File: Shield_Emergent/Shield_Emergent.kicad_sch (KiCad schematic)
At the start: 18 parts, among them J1 Conn_01x02_Female, J3 Conn_01x02_Female, J5 Conn_02x06_Odd_Even, U1 Raspberri_Pi_Pico, U2 TPS2553, U3 TPS2553

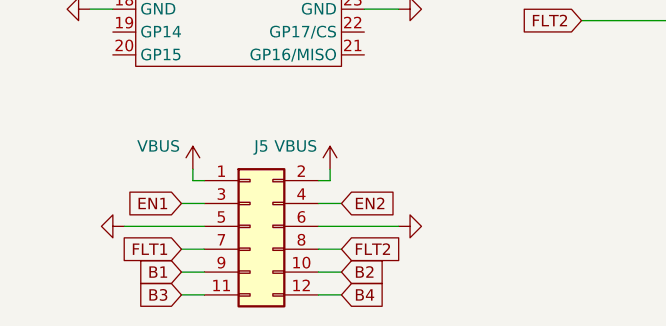
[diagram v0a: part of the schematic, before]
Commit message: v1.7 DRC was conducted
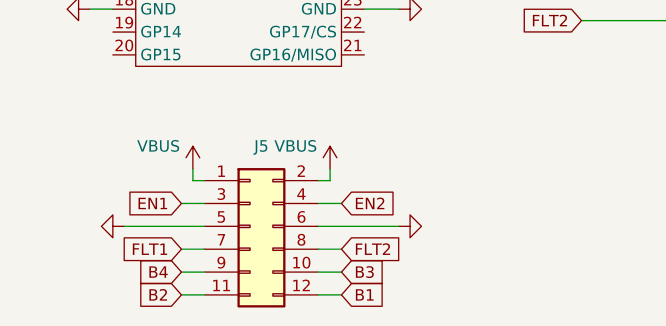
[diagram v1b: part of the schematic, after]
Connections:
- net B1: now also J5.12 (Pin_12); no longer J5.9 (Pin_9)
- net B2: now also J5.11 (Pin_11); no longer J5.10 (Pin_10)
- net B3: now also J5.10 (Pin_10); no longer J5.11 (Pin_11)
- net B4: now also J5.9 (Pin_9); no longer J5.12 (Pin_12)
